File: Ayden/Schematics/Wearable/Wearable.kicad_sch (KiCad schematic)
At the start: 6 parts

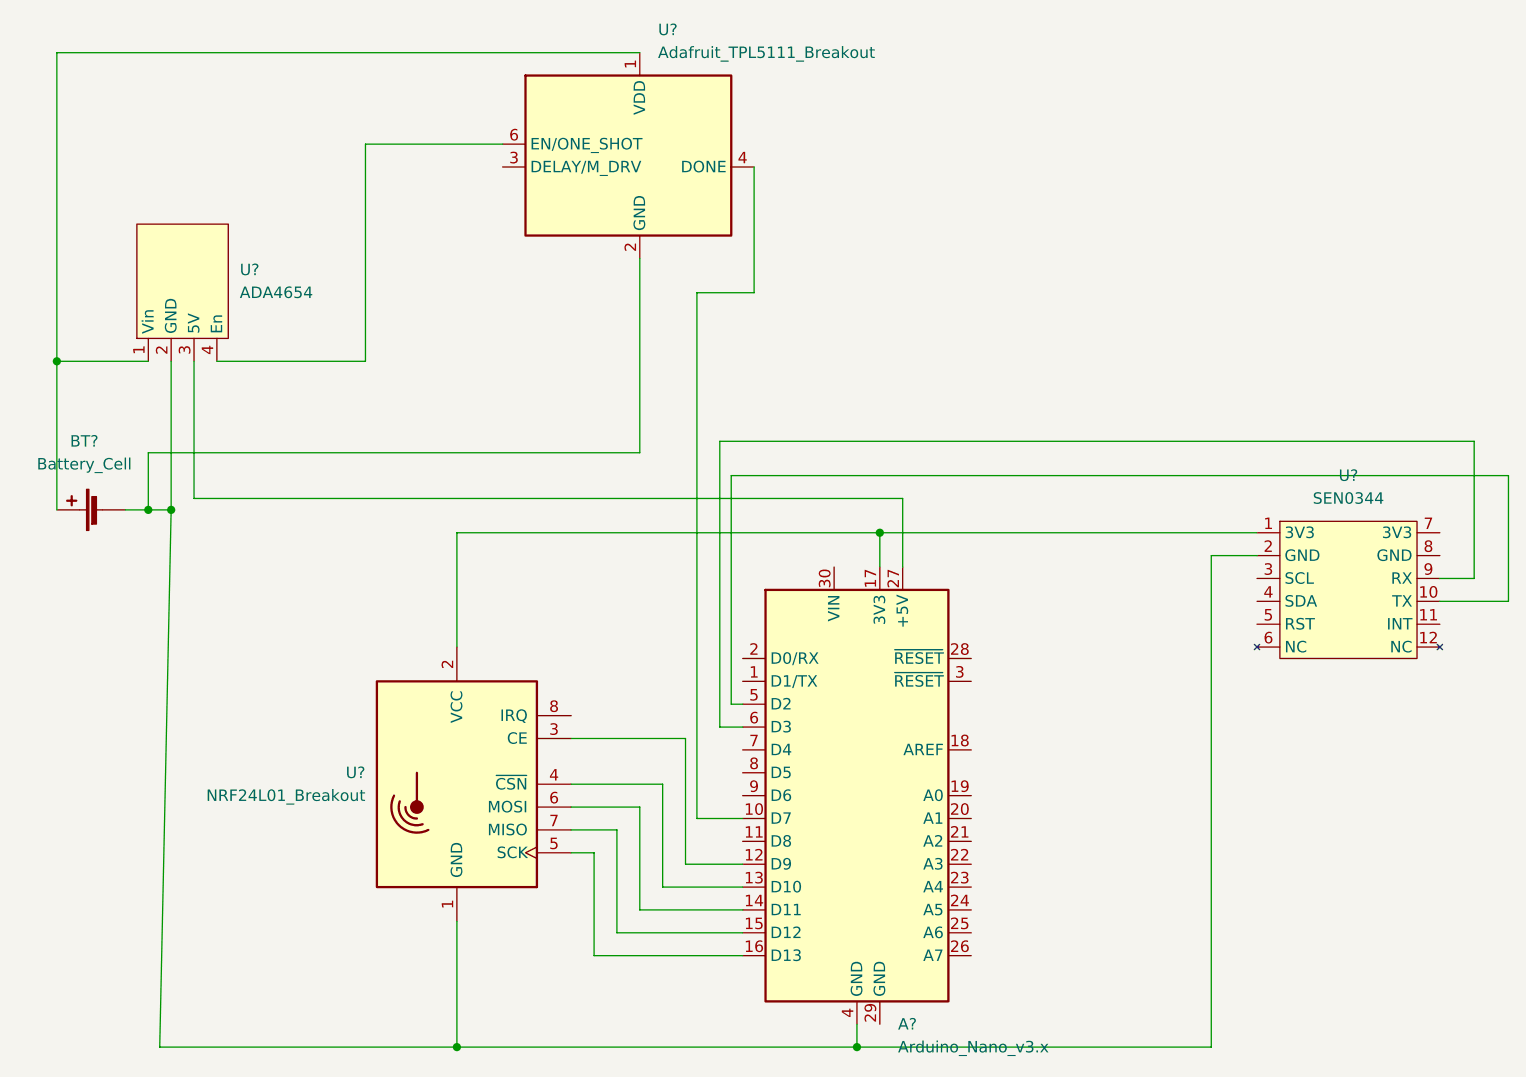
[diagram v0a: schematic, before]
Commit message: Organized schematic for project demo
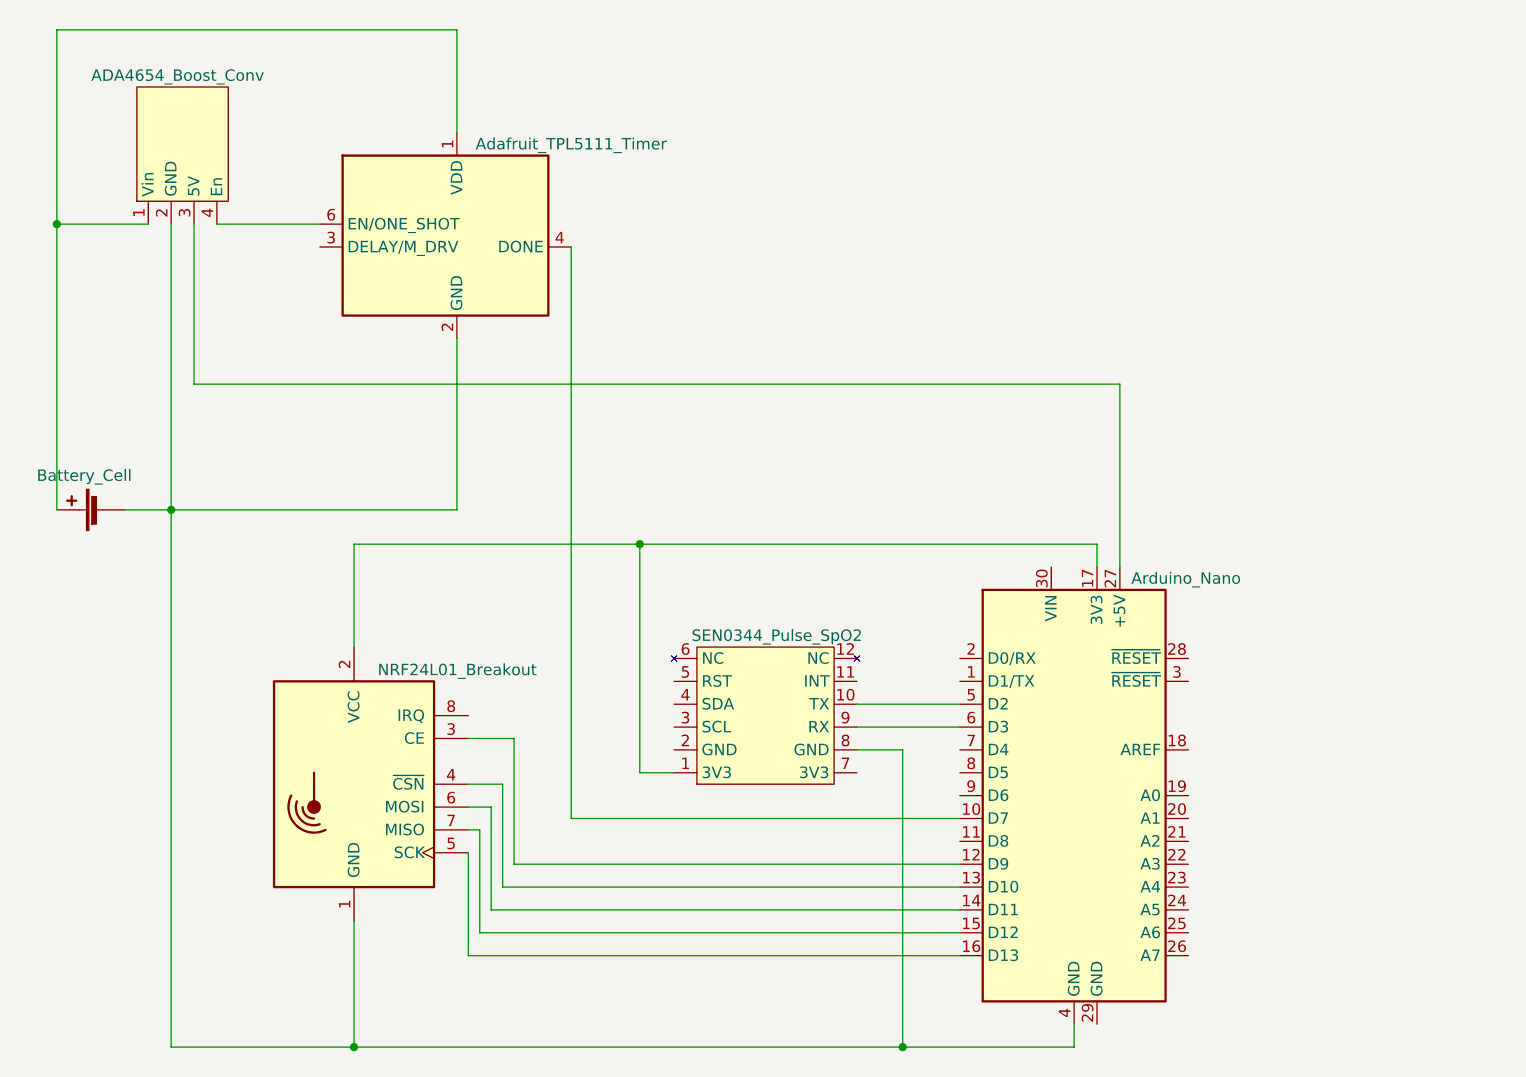
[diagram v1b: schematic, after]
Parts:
- A1: renamed from A?; value Arduino_Nano_v3.x -> Arduino_Nano
- U?: value ADA4654 -> ADA4654_Boost_Conv
- U?: value SEN0344 -> SEN0344_Pulse_SpO2
- U?: value Adafruit_TPL5111_Breakout -> Adafruit_TPL5111_Timer
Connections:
- net at A1.4 (GND), BT?.2 (-), U?.1 (GND)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: now also U?.8 (GND); no longer U?.2 (GND)
